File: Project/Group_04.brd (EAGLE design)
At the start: 71.1 x 56.9 mm, 29 parts, among them J1 POWER_JACKPTH_LOCK, U1 +12v

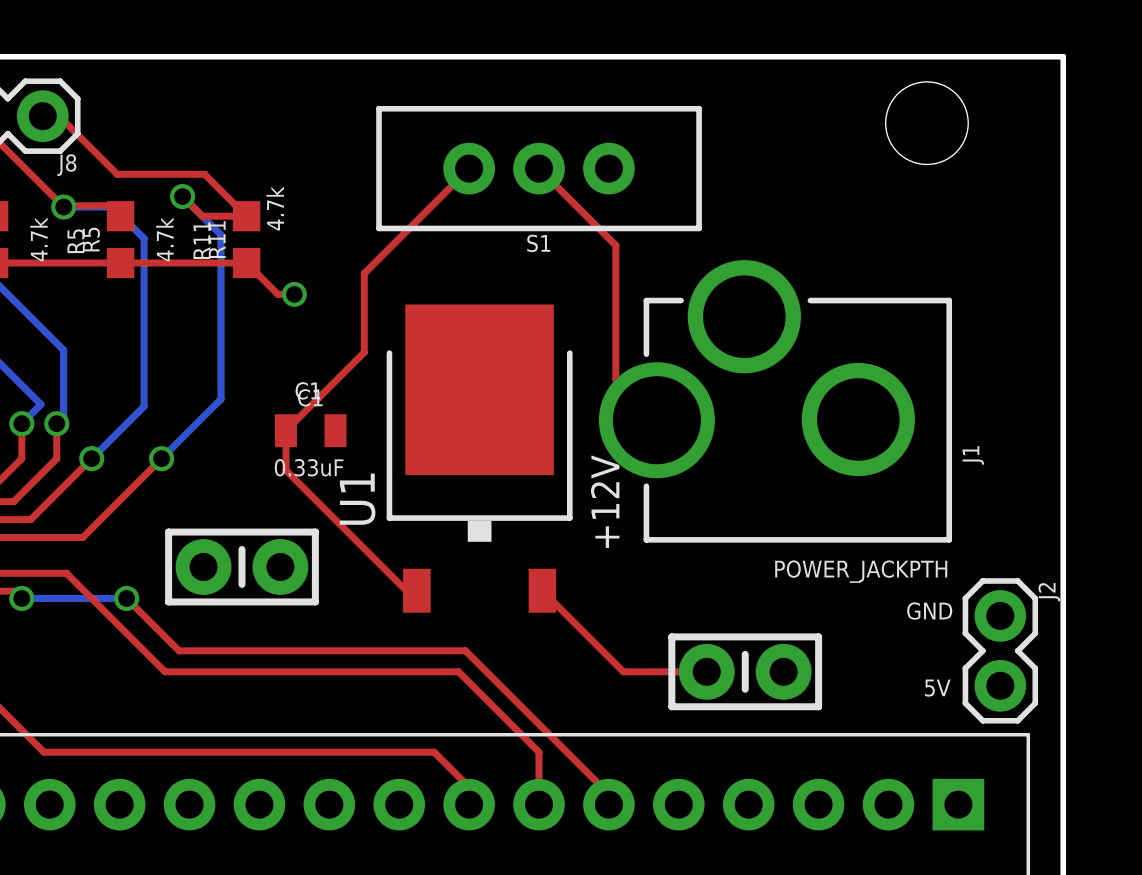
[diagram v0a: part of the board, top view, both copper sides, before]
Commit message: Final version
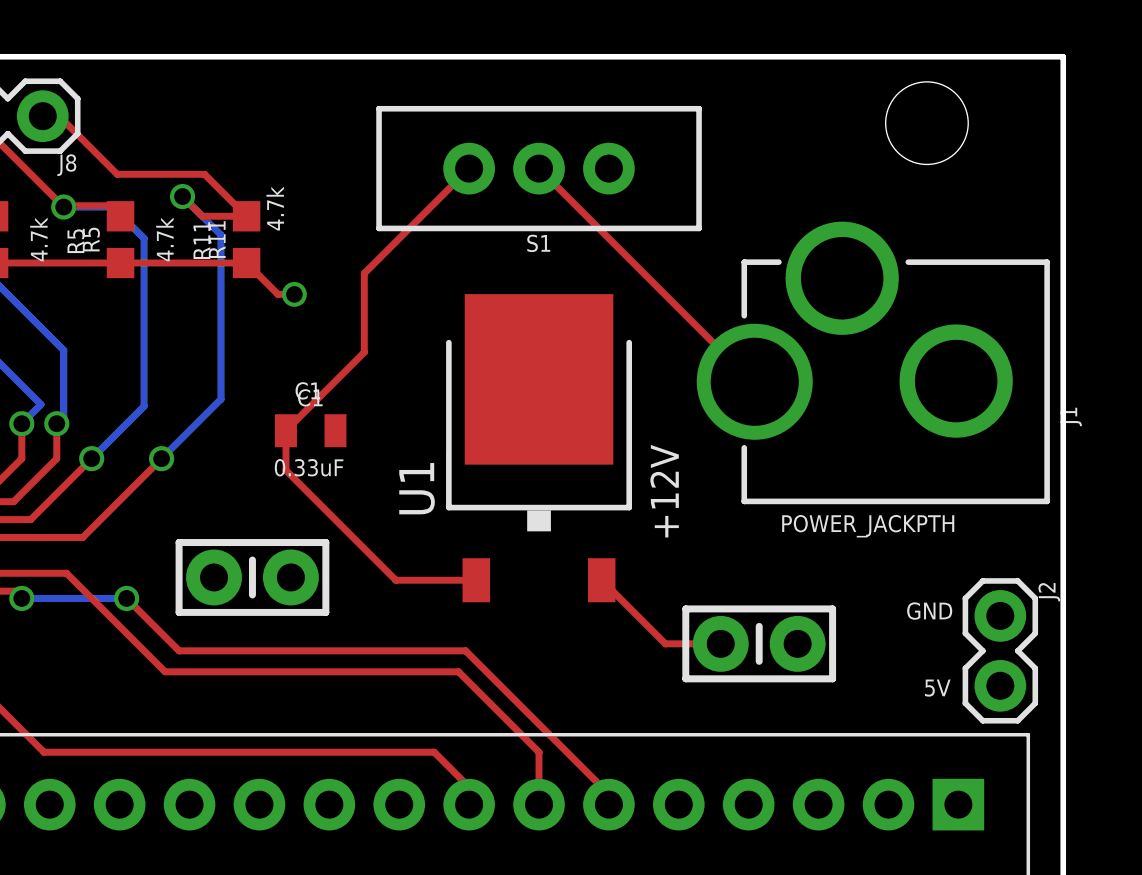
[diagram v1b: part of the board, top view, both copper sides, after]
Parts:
- moved J1 3.82 mm to (73.8, 45.1)
- moved U1 2.19 mm to (52.1, 42.7)
- moved C3 1.14 mm to (60.1, 35.6)
- moved C2 0.54 mm to (41.7, 38.0)
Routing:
- net 12V: track 20.3 -> 22.3 mm
- net 5V: track 46.3 -> 44.4 mm
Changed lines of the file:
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@@
 <text x="25.146" y="42.799" size="0.6096" layer="21">TCA9546ASMD</text>
 <text x="12.573" y="36.195" size="0.6096" layer="21" rot="R90">TMUX1208</text>
-<text x="53.975" y="42.418" size="1.016" layer="21" rot="R270">+12V</text>
+<text x="56.134" y="42.799" size="1.016" layer="21" rot="R270">+12V</text>
 <text x="9.398" y="49.41983125" size="0.6096" layer="21" rot="R90">4.7k</text>
 <text x="42.418" y="41.656" size="0.6096" layer="21">0.33uF</text>
 <text x="66.04" y="33.655" size="0.6096" layer="21">5V</text>
 <text x="65.405" y="36.449" size="0.6096" layer="21">GND</text>
-<text x="60.579" y="37.973" size="0.6096" layer="21">POWER_JACKPTH</text>
+<text x="60.833" y="39.624" size="0.6096" layer="21">POWER_JACKPTH</text>
 <text x="43.18" y="44.45" size="0.6096" layer="21">C1</text>
 <text x="13.977234375" y="49.41983125" size="0.6096" layer="21" rot="R90">4.7k</text>
@@
 <attribute name="VALUE" x="43.7729375" y="42.418" size="0.6096" layer="27" font="vector" ratio="20" align="top-center"/>
 </element>
-<element name="C2" library="SparkFun-Capacitors" package="CAP-PTH-SMALL-KIT" value="0.1uF" x="41.275" y="38.354" smashed="yes" rot="R180">
-<attribute name="PROD_ID" value="CAP-08370" x="-17.145" y="95.504" size="1.778" layer="27" rot="R180" display="off"/>
-</element>
-<element name="C3" library="SparkFun-Capacitors" package="CAP-PTH-SMALL-KIT" value="0.1uF" x="59.563" y="34.544" smashed="yes">
-<attribute name="PROD_ID" value="CAP-08370" x="124.333" y="-22.606" size="1.778" layer="27" display="off"/>
+<element name="C2" library="SparkFun-Capacitors" package="CAP-PTH-SMALL-KIT" value="0.1uF" x="41.656" y="37.973" smashed="yes" rot="R180">
+<attribute name="PROD_ID" value="CAP-08370" x="-16.764" y="95.123" size="1.778" layer="27" rot="R180" display="off"/>
+</element>
+<element name="C3" library="SparkFun-Capacitors" package="CAP-PTH-SMALL-KIT" value="0.1uF" x="60.071" y="35.56" smashed="yes">
+<attribute name="PROD_ID" value="CAP-08370" x="124.841" y="-21.59" size="1.778" layer="27" display="off"/>
 </element>
 <element name="D1" library="SparkFun-LED" package="LED-1206" value="BLUE" x="10.287" y="3.682953125" smashed="yes">
@@
 <attribute name="VALUE" x="10.287" y="2.730453125" size="0.6096" layer="27" font="vector" ratio="20" align="top-center"/>
 </element>
-<element name="J1" library="SparkFun-Connectors" package="POWER_JACK_PTH_LOCK" value="POWER_JACKPTH_LOCK" x="70.231" y="43.688" smashed="yes" rot="R90">
-<attribute name="NAME" x="68.072" y="42.1132" size="0.6096" layer="25" font="vector" ratio="20" rot="R90"/>
-<attribute name="PROD_ID" value="CONN-08197" x="98.171" y="64.008" size="1.778" layer="27" rot="R90" display="off"/>
-<attribute name="SF_ID" value="PRT-00119" x="98.171" y="64.008" size="1.778" layer="27" rot="R90" display="off"/>
-<attribute name="VALUE" x="69.088" y="41.783" size="0.6096" layer="27" font="vector" ratio="20" rot="R90"/>
+<element name="J1" library="SparkFun-Connectors" package="POWER_JACK_PTH_LOCK" value="POWER_JACKPTH_LOCK" x="73.787" y="45.085" smashed="yes" rot="R90">
+<attribute name="NAME" x="71.628" y="43.5102" size="0.6096" layer="25" font="vector" ratio="20" rot="R90"/>
+<attribute name="PROD_ID" value="CONN-08197" x="101.727" y="65.405" size="1.778" layer="27" rot="R90" display="off"/>
+<attribute name="SF_ID" value="PRT-00119" x="101.727" y="65.405" size="1.778" layer="27" rot="R90" display="off"/>
+<attribute name="VALUE" x="72.644" y="43.18" size="0.6096" layer="27" font="vector" ratio="20" rot="R90"/>
 </element>
 <element name="J2" library="SparkFun-Connectors" package="1X02" value="" x="68.834" y="36.576" smashed="yes" rot="R270">
@@
 </element>
 <element name="U$3" library="CY8KIT-059" package="CY8CKIT-059_TARGET" value="CY8CKIT-059_TARGET" x="36.83" y="20.828" smashed="yes"/>
-<element name="U1" library="SparkFun-IC-Power" package="TO-252" value="+12v" x="49.911" y="42.291" smashed="yes">
-<attribute name="NAME" x="46.101" y="39.751" size="1.27" layer="25" rot="R90"/>
-<attribute name="PROD_ID" value="VREG-12370" x="88.011" y="9.271" size="1.778" layer="27" display="off"/>
-<attribute name="VALUE" x="54.991" y="39.751" size="1.27" layer="27" rot="R90"/>
+<element name="U1" library="SparkFun-IC-Power" package="TO-252" value="+12v" x="52.07" y="42.672" smashed="yes">
+<attribute name="NAME" x="48.26" y="40.132" size="1.27" layer="25" rot="R90"/>
+<attribute name="PROD_ID" value="VREG-12370" x="90.17" y="9.652" size="1.778" layer="27" display="off"/>
+<attribute name="VALUE" x="57.15" y="40.132" size="1.27" layer="27" rot="R90"/>
 </element>
 <element name="U2" library="SparkFun-Sensors" package="TO-92" value="" x="40.6929125" y="3.682996875" smashed="yes" rot="R90">
@@
 <vertex x="0" y="56.896"/>
 <vertex x="0" y="0"/>
-<vertex x="0" y="0"/>
 <vertex x="71.12" y="0"/>
 <vertex x="71.12" y="56.896"/>
@@
 <contactref element="J1" pad="PWR"/>
 <contactref element="S1" pad="2"/>
-<wire x1="56.3532" y1="43.688" x2="54.864" y2="45.1772" width="0.254" layer="1"/>
-<wire x1="54.864" y1="50.038" x2="52.07" y2="52.832" width="0.254" layer="1"/>
-<wire x1="54.864" y1="45.1772" x2="54.864" y2="50.038" width="0.254" layer="1"/>
+<wire x1="59.9092" y1="45.085" x2="59.817" y2="45.085" width="0.254" layer="1"/>
+<wire x1="59.817" y1="45.085" x2="52.07" y2="52.832" width="0.254" layer="1"/>
 </signal>
 <signal name="12V">
@@
 <contactref element="C1" pad="1"/>
 <contactref element="U1" pad="1"/>
-<wire x1="47.631" y1="37.491" x2="47.25" y2="37.491" width="0.254" layer="1"/>
-<wire x1="47.25" y1="37.491" x2="42.8729375" y2="41.8680625" width="0.254" layer="1"/>
+<wire x1="49.79" y1="37.872" x2="46.869" y2="37.872" width="0.254" layer="1"/>
+<wire x1="46.869" y1="37.872" x2="42.8729375" y2="41.8680625" width="0.254" layer="1"/>
 <wire x1="42.8729375" y1="43.307" x2="42.8729375" y2="41.8680625" width="0.254" layer="1"/>
 <wire x1="45.72" y1="46.1540625" x2="42.8729375" y2="43.307" width="0.254" layer="1"/>
@@
 <wire x1="19.875946875" y1="49.3999375" x2="15.2967125" y2="49.3999375" width="0.254" layer="1"/>
 <wire x1="15.2967125" y1="49.3999375" x2="10.717478125" y2="49.3999375" width="0.254" layer="1"/>
-<wire x1="52.191" y1="37.491" x2="55.138" y2="34.544" width="0.254" layer="1"/>
-<wire x1="55.138" y1="34.544" x2="58.166" y2="34.544" width="0.254" layer="1"/>
+<wire x1="54.35" y1="37.872" x2="56.662" y2="35.56" width="0.254" layer="1"/>
+<wire x1="56.662" y1="35.56" x2="58.674" y2="35.56" width="0.254" layer="1"/>
 <polygon width="0.254" layer="16" isolate="0.3048">
 <vertex x="0" y="56.896"/>
 <vertex x="0" y="0"/>
-<vertex x="0" y="0"/>
 <vertex x="71.12" y="0"/>
